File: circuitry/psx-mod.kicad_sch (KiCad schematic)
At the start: 57 parts, among them J1 2x3P, J2 1x6P, J3 1x6P, J4 1x6P, J5 USB 2.0 Type-C, Q1 SI2302, Q2 SI2302, SW1 RESET, U1 TPS78318DDCT, U2 CDCE925PWR, U3 74HC04, U4 ATmega328P-A, U5 USBLC6-2SC6, U6 CH340G, Y1 16MHz, Y2 27MHz, Y3 12MHz

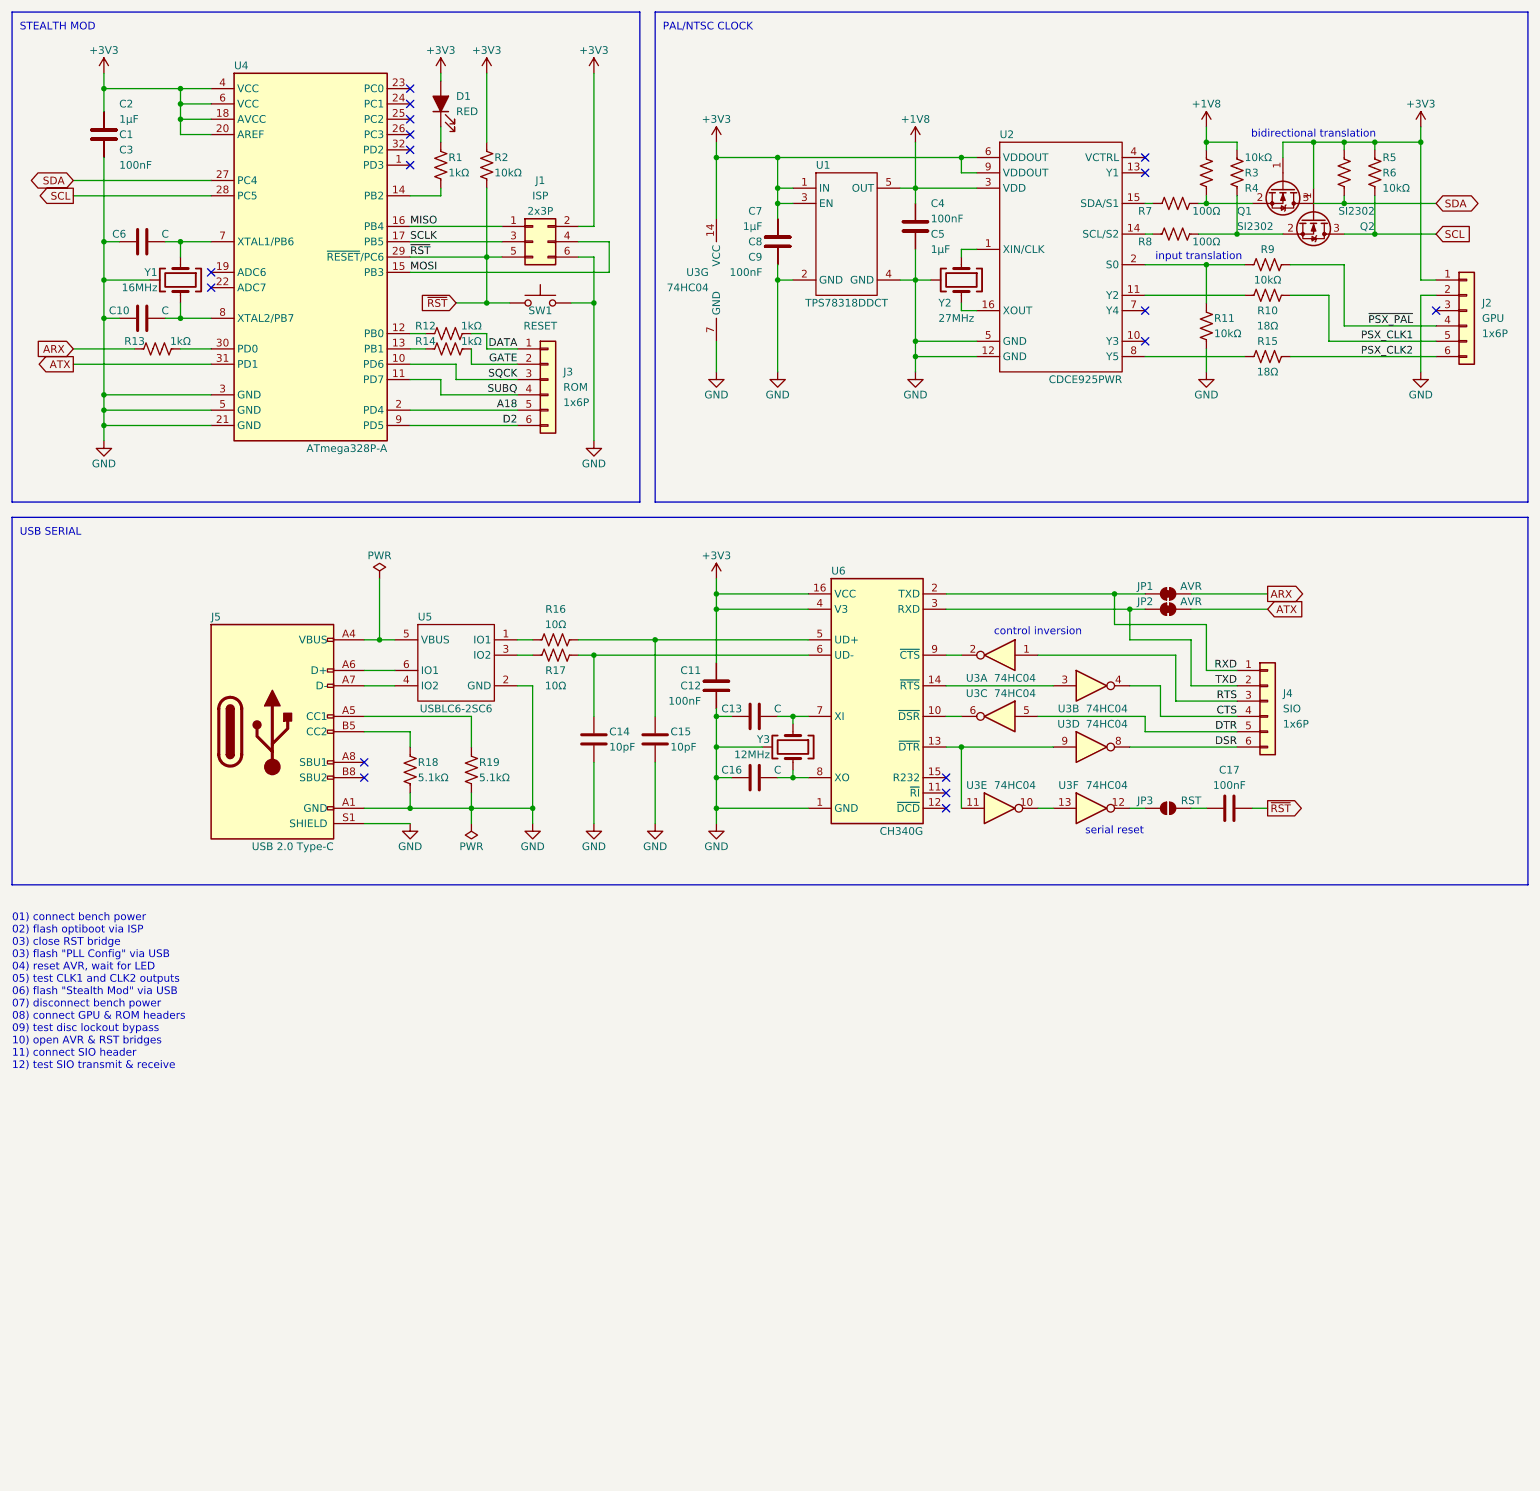
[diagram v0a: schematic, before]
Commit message: Completed schematic and layout (badly).
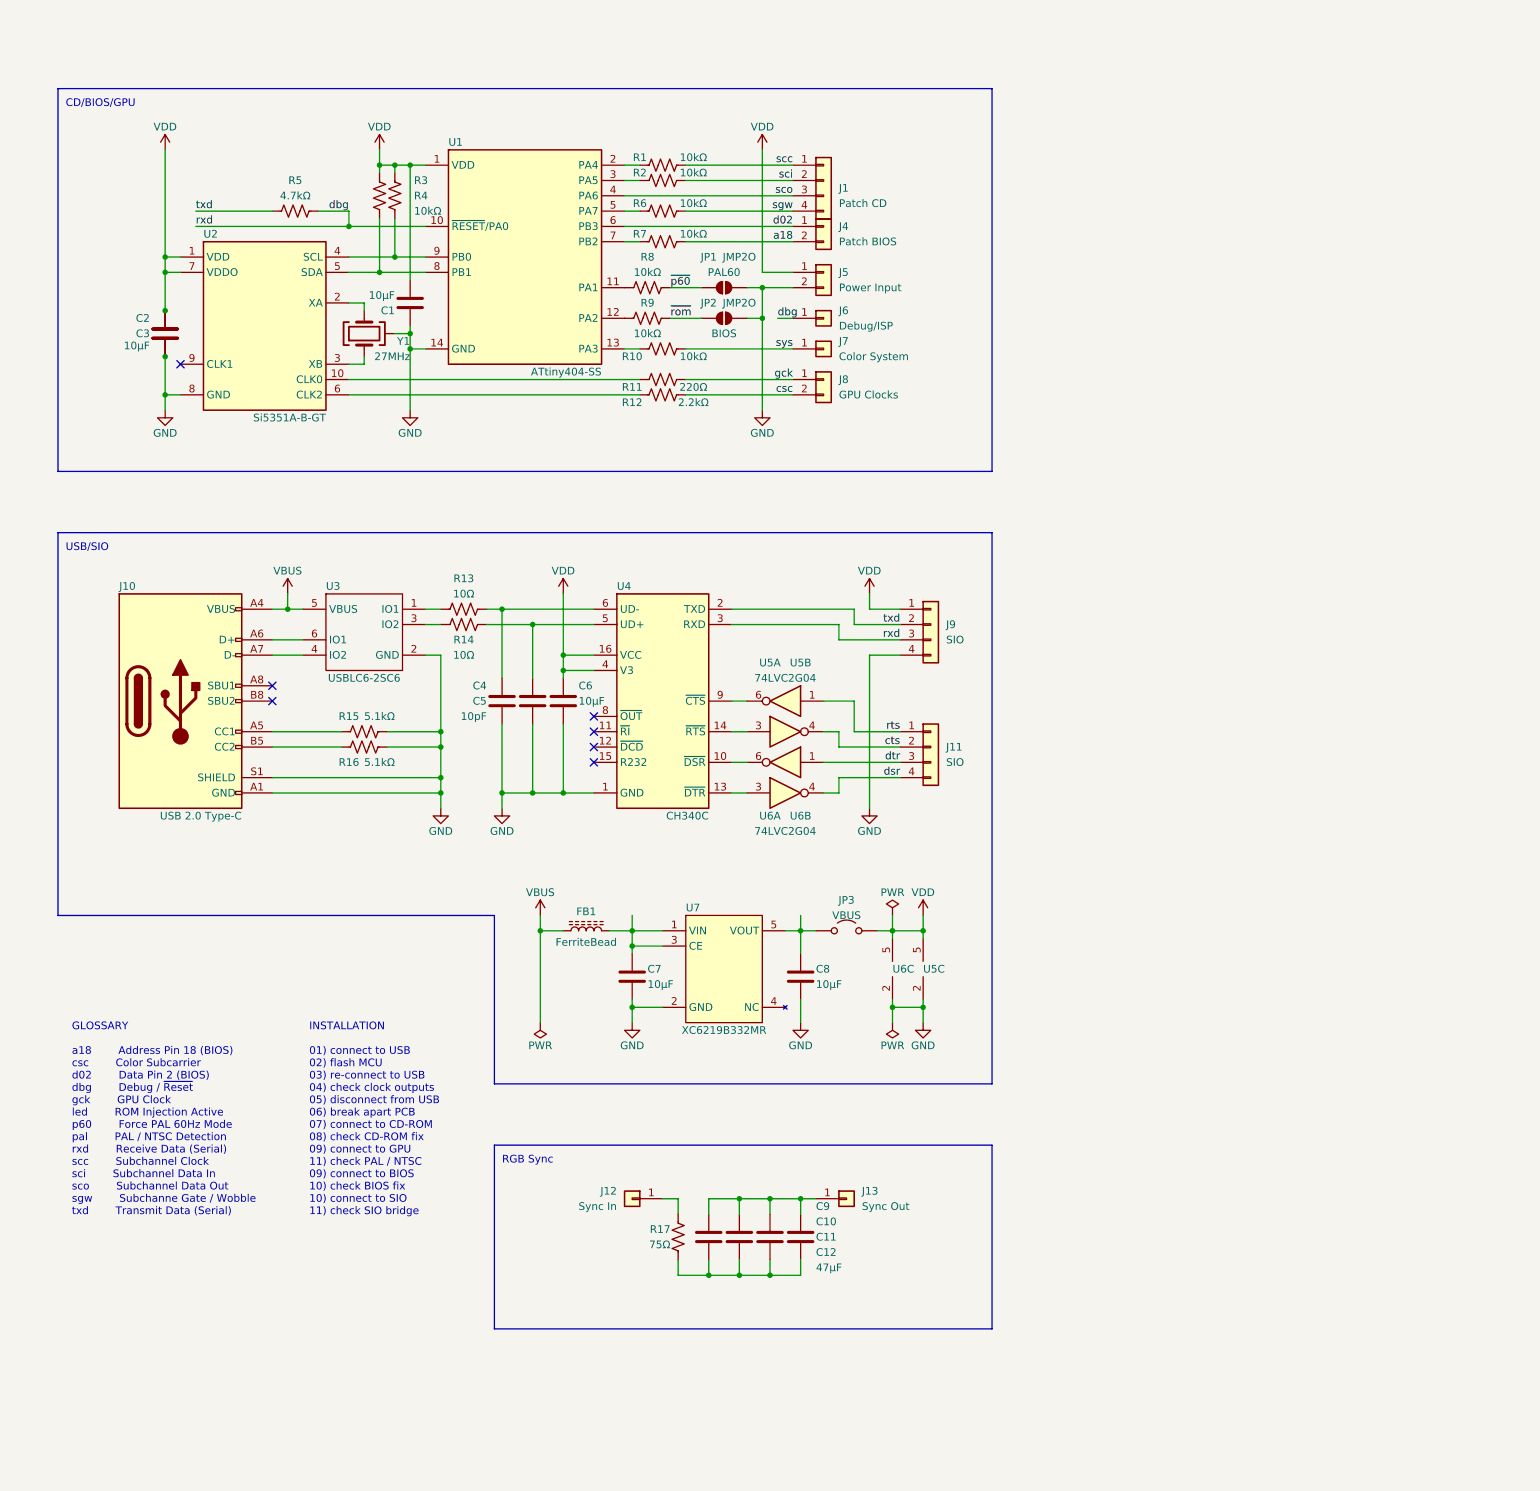
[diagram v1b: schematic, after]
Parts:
- removed C13, C16: C, Capacitor_SMD:C_0805_2012Metric_Pad1.18x1.45mm_HandSolder, symbol Device:C
- removed C14, C15: 10pF, Capacitor_SMD:C_0805_2012Metric_Pad1.18x1.45mm_HandSolder, symbol Device:C
- removed C17: 100nF, Capacitor_SMD:C_0805_2012Metric_Pad1.18x1.45mm_HandSolder, symbol Device:C
- removed D1: RED, Capacitor_SMD:C_0805_2012Metric_Pad1.18x1.45mm_HandSolder, symbol Device:LED_Filled
- removed J1: 2x3P, PSX_Mod:CONN-SMD_POGO-ISP, symbol Connector_Generic:Conn_02x03_Odd_Even
- removed J2, J3, J4: 1x6P, PSX_Mod:CONN-PH 1x06_P2.00mm_Horizontal, symbol Connector_Generic:Conn_01x06
- removed J5: USB 2.0 Type-C, PSX_Mod:CONN-SMD_HX-TYPE-C-16PIN, symbol PSX_Mod:USB_C_Receptacle_USB2.0_16P
- removed JP1, JP2: SolderJumper_2_Bridged, Jumper:SolderJumper-2_P1.3mm_Bridged2Bar_RoundedPad1.0x1.5mm, symbol Jumper:SolderJumper_2_Bridged
- removed JP3: SolderJumper_2_Open, Jumper:SolderJumper-2_P1.3mm_Open_RoundedPad1.0x1.5mm, symbol Jumper:SolderJumper_2_Open
- removed Q1, Q2: SI2302, Package_TO_SOT_SMD:SOT-23_Handsoldering, symbol Ashlyns_Symbols:SI2302
- removed R18, R19: 5.1kΩ, Resistor_SMD:R_0805_2012Metric_Pad1.20x1.40mm_HandSolder, symbol Device:R_US
- removed SW1: RESET, Button_Switch_SMD:SW_Push_1P1T_NO_6x6mm_H9.5mm, symbol Switch:SW_Push
- removed U1: TPS78318DDCT, Package_TO_SOT_SMD:SOT-23-5, symbol PSX_Mod:TPS78318DDCT
- removed U2: CDCE925PWR, Package_SO:TSSOP-16_4.4x5mm_P0.65mm, symbol PSX_Mod:CDCE925PWR
- removed U3: 74HC04, Package_SO:SOIC-14_3.9x8.7mm_P1.27mm, symbol PSX_Mod:74HC04
- removed U4: ATmega328P-A, Package_QFP:TQFP-32_7x7mm_P0.8mm, symbol PSX_Mod:ATmega328P-A
- removed U5: USBLC6-2SC6, Package_TO_SOT_SMD:SOT-23-6, symbol PSX_Mod:USBLC6_2SC6
- removed U6: CH340G, Package_SO:SOIC-16_3.9x9.9mm_P1.27mm, symbol PSX_Mod:CH340G
- removed Y2: 27MHz, Crystal:Crystal_SMD_3225-4Pin_3.2x2.5mm_HandSoldering, symbol PSX_Mod:Crystal
- removed Y3: 12MHz, Crystal:Crystal_SMD_3225-4Pin_3.2x2.5mm_HandSoldering, symbol PSX_Mod:Crystal
- added FB1: FerriteBead, Inductor_SMD:L_1206_3216Metric_Pad1.42x1.75mm_HandSolder, symbol Device:L_Ferrite
- added J1, J11, J9: Conn_01x04, PSX_Mod:CONN-SMD_4P, symbol Connector_Generic:Conn_01x04
- added J10: USB 2.0 Type-C, PSX_Mod:CONN-SMD_HX-TYPE-C-16PIN, symbol PSX_Mod:USB_C_Receptacle_USB2.0_16P
- added J12, J13, J6, J7: Conn_01x01, PSX_Mod:CONN-SMD_1P, symbol Connector_Generic:Conn_01x01
- added J4, J5, J8: Conn_01x02, PSX_Mod:CONN-SMD_2P, symbol Connector_Generic:Conn_01x02
- added JP1, JP2: JMP2O, Jumper:SolderJumper-2_P1.3mm_Open_RoundedPad1.0x1.5mm, symbol Jumper:SolderJumper_2_Open
- added JP3: Jumper_2_Open, Jumper:SolderJumper-2_P1.3mm_Open_RoundedPad1.0x1.5mm, symbol Jumper:Jumper_2_Open
- added U1: ATtiny404-SS, Package_SO:SOIC-14_3.9x8.7mm_P1.27mm, symbol PSX_Mod:ATtiny404-SS
- added U2: Si5351A-B-GT, Package_SO:MSOP-10_3x3mm_P0.5mm, symbol PSX_Mod:Si5351A-B-GT
- added U3: USBLC6-2SC6, Package_TO_SOT_SMD:SOT-23-6, symbol PSX_Mod:USBLC6_2SC6
- added U4: CH340C, Package_SO:SOIC-16_3.9x9.9mm_P1.27mm, symbol PSX_Mod:CH340C
- added U5, U6: 74LVC2G04, Package_TO_SOT_SMD:SOT-23-6, symbol PSX_Mod:74LVC2G04
- added U7: XC6219B332MR, Package_TO_SOT_SMD:SOT-23-5, symbol PSX_Mod:XC6219B332MR
- C1: value 100nF -> 10µF; footprint Capacitor_SMD:C_0805_2012Metric_Pad1.18x1.45mm_HandSolder -> Capacitor_SMD:C_0603_1608Metric_Pad1.08x0.95mm_HandSolder
- C10: value C -> 47µF; footprint Capacitor_SMD:C_0805_2012Metric_Pad1.18x1.45mm_HandSolder -> Capacitor_SMD:C_1206_3216Metric_Pad1.33x1.80mm_HandSolder
- C11: value 100nF -> 47µF; footprint Capacitor_SMD:C_0805_2012Metric_Pad1.18x1.45mm_HandSolder -> Capacitor_SMD:C_1206_3216Metric_Pad1.33x1.80mm_HandSolder; Proximity USB -> (none)
- C12: value 100nF -> 47µF; footprint Capacitor_SMD:C_0805_2012Metric_Pad1.18x1.45mm_HandSolder -> Capacitor_SMD:C_1206_3216Metric_Pad1.33x1.80mm_HandSolder; Proximity Inverter -> (none)
- C2: value 1µF -> 10µF; footprint Capacitor_SMD:C_0805_2012Metric_Pad1.18x1.45mm_HandSolder -> Capacitor_SMD:C_0603_1608Metric_Pad1.08x0.95mm_HandSolder; Proximity (none) -> PLL
- C3: value 100nF -> 10µF; footprint Capacitor_SMD:C_0805_2012Metric_Pad1.18x1.45mm_HandSolder -> Capacitor_SMD:C_0603_1608Metric_Pad1.08x0.95mm_HandSolder; Proximity (none) -> PLL
- C4: value 100nF -> 10pF; footprint Capacitor_SMD:C_0805_2012Metric_Pad1.18x1.45mm_HandSolder -> Capacitor_SMD:C_0603_1608Metric_Pad1.08x0.95mm_HandSolder; Proximity PLL -> (none)
- C5: value 1µF -> 10pF; footprint Capacitor_SMD:C_0805_2012Metric_Pad1.18x1.45mm_HandSolder -> Capacitor_SMD:C_0603_1608Metric_Pad1.08x0.95mm_HandSolder; Proximity VREG -> (none)
- C6: value C -> 10µF; footprint Capacitor_SMD:C_0805_2012Metric_Pad1.18x1.45mm_HandSolder -> Capacitor_SMD:C_0603_1608Metric_Pad1.08x0.95mm_HandSolder
- C7: value 1µF -> 10µF; footprint Capacitor_SMD:C_0805_2012Metric_Pad1.18x1.45mm_HandSolder -> Capacitor_SMD:C_0603_1608Metric_Pad1.08x0.95mm_HandSolder; Proximity VREG -> (none)
- C8: value 100nF -> 10µF; footprint Capacitor_SMD:C_0805_2012Metric_Pad1.18x1.45mm_HandSolder -> Capacitor_SMD:C_0603_1608Metric_Pad1.08x0.95mm_HandSolder; Proximity PLL -> (none)
- C9: value 100nF -> 47µF; footprint Capacitor_SMD:C_0805_2012Metric_Pad1.18x1.45mm_HandSolder -> Capacitor_SMD:C_1206_3216Metric_Pad1.33x1.80mm_HandSolder; Proximity PLL -> (none)
- R1: value 1kΩ -> 10kΩ; footprint Resistor_SMD:R_0805_2012Metric_Pad1.20x1.40mm_HandSolder -> Resistor_SMD:R_0603_1608Metric_Pad0.98x0.95mm_HandSolder
- R10: value 18Ω -> 10kΩ; footprint Resistor_SMD:R_0805_2012Metric_Pad1.20x1.40mm_HandSolder -> Resistor_SMD:R_0603_1608Metric_Pad0.98x0.95mm_HandSolder
- R11: value 10kΩ -> 220Ω; footprint Resistor_SMD:R_0805_2012Metric_Pad1.20x1.40mm_HandSolder -> Resistor_SMD:R_0603_1608Metric_Pad0.98x0.95mm_HandSolder
- R12: value 1kΩ -> 2.2kΩ; footprint Resistor_SMD:R_0805_2012Metric_Pad1.20x1.40mm_HandSolder -> Resistor_SMD:R_0603_1608Metric_Pad0.98x0.95mm_HandSolder
- R13, R14: value 1kΩ -> 10Ω; footprint Resistor_SMD:R_0805_2012Metric_Pad1.20x1.40mm_HandSolder -> Resistor_SMD:R_0603_1608Metric_Pad0.98x0.95mm_HandSolder
- R15: value 18Ω -> 5.1kΩ; footprint Resistor_SMD:R_0805_2012Metric_Pad1.20x1.40mm_HandSolder -> Resistor_SMD:R_0603_1608Metric_Pad0.98x0.95mm_HandSolder
- R16: value 10Ω -> 5.1kΩ; footprint Resistor_SMD:R_0805_2012Metric_Pad1.20x1.40mm_HandSolder -> Resistor_SMD:R_0603_1608Metric_Pad0.98x0.95mm_HandSolder
- R17: value 10Ω -> 75Ω; footprint Resistor_SMD:R_0805_2012Metric_Pad1.20x1.40mm_HandSolder -> Resistor_SMD:R_1206_3216Metric_Pad1.30x1.75mm_HandSolder
- R2, R3, R4, R6, R9: footprint Resistor_SMD:R_0805_2012Metric_Pad1.20x1.40mm_HandSolder -> Resistor_SMD:R_0603_1608Metric_Pad0.98x0.95mm_HandSolder
- R5: value 10kΩ -> 4.7kΩ; footprint Resistor_SMD:R_0805_2012Metric_Pad1.20x1.40mm_HandSolder -> Resistor_SMD:R_0603_1608Metric_Pad0.98x0.95mm_HandSolder
- R7, R8: value 100Ω -> 10kΩ; footprint Resistor_SMD:R_0805_2012Metric_Pad1.20x1.40mm_HandSolder -> Resistor_SMD:R_0603_1608Metric_Pad0.98x0.95mm_HandSolder
- Y1: value 16MHz -> 27MHz; footprint Crystal:Crystal_SMD_3225-4Pin_3.2x2.5mm_HandSoldering -> Crystal:Crystal_SMD_3225-4Pin_3.2x2.5mm; Load (none) -> 10pF
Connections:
- net PSX_CLK2 is gone; now on net GND: R15.2
- net GND: now also C6.2, R16.2, J10.A1 (GND), J10.A12 (GND), J10.B1 (GND), J10.B12 (GND), J10.S1 (SHIELD), J5.2 (Pin_2), J9.4 (Pin_4), JP1.2 (B), JP2.2 (B), U1.14 (GND), U2.8 (GND), U3.2 (GND), U4.1 (GND), U5.2 (GND), U6.2 (GND), U7.2 (GND); no longer C10.1, C11.2, C12.2, C6.1, C9.2, R11.2
- net at R10.1: now also U1.13 (PA3)
- net at R11.1: now also U2.10 (CLK0); no longer R9.1
- net at R12.1: now also U2.6 (CLK2)
- net at R14.1: now also U3.3 (IO2)
- net scc: now reaches R1.2
- net scc: now also J1.1 (Pin_1)
- net at R13.2: now also C4.1, U4.6 (UD-)
- net at Y1.1: now also U2.3 (XB); no longer C6.2
- net at C10.2: now also C11.2, C12.2, C9.2, R17.1; no longer Y1.3
- net at R7.1: now also U1.7 (PB2)
- net at R3.2: now also U1.8 (PB1), U2.5 (SDA); no longer R7.2
- net at R8.1: now also U1.11 (PA1)
- net at R4.2: now also U1.9 (PB0), U2.4 (SCL); no longer R8.2
- net at R1.1: now also U1.2 (PA4)
- net at R15.1: now also J10.A5 (CC1)
- net at R16.1: now also J10.B5 (CC2)
- net at R17.2: now also J12.1 (Pin_1)
- net +1V8 renamed VDD
- net VDD: now also C1.1, C2.1, C3.1, C6.1, J5.1 (Pin_1), J9.1 (Pin_1), JP3.2 (B), U1.1 (VDD), U2.1 (VDD), U2.7 (VDDO), U4.16 (VCC), U4.4 (V3), U5.5 (VCC), U6.5 (VCC); no longer C4.1, C5.1
- removed net +3V3: C1.1, C11.1, C12.1, C2.1, C3.1, C7.1, C8.1, C9.1, R2.1, R5.1, R6.1
- net ARX: no longer names the net of R13.1
- net ARX: now also U3.1 (IO1)
- net DATA renamed csc
- net csc: now also J8.2 (Pin_2)
- net GATE: no longer names the net of R14.2
- net GATE: now also C5.1, U4.5 (UD+)
- net PSX_CLK1 renamed sys
- net sys: now also J7.1 (Pin_1)
- net SCL renamed sgw
- net sgw: now also J1.4 (Pin_4)
- net SDA renamed dbg
- net dbg: now also J6.1 (Pin_1), J9.3 (Pin_3), U1.10 (~{RESET}/PA0), U4.3 (RXD)
- net ~{PSX_PAL} renamed ~{rom}
- net ~{rom}: now also JP2.1 (A)
- net ~{RST} renamed sci
- net sci: now also J1.2 (Pin_2)
- new net: U4.10 (~{DSR}), U6.6 (~{Y1})
- new net: U4.13 (~{DTR}), U6.3 (A2)
- new net: U4.14 (~{RTS}), U5.3 (A2)
- new net: U4.9 (~{CTS}), U5.6 (~{Y1})
- new net: C10.1, C11.1, C12.1, C9.1, J13.1 (Pin_1)
- new net: C7.1, FB1.2, U7.1 (VIN), U7.3 (CE)
- new net: C8.1, JP3.1 (A), U7.5 (VOUT)
- new net: R9.1, U1.12 (PA2)
- new net: R2.1, U1.3 (PA5)
- new net: R6.1, U1.5 (PA7)
- new net: J10.A7 (D-), J10.B7 (D-), U3.4 (IO2)
- new net: J10.A6 (D+), J10.B6 (D+), U3.6 (IO1)
- new net: U2.2 (XA), Y1.3
- new net VBUS: FB1.1, J10.A4 (VBUS), J10.A9 (VBUS), J10.B4 (VBUS), J10.B9 (VBUS), U3.5 (VBUS)
- new net a18: J4.2 (Pin_2), R7.2
- new net cts: J11.2 (Pin_2), U5.4 (~{Y2})
- new net d02: J4.1 (Pin_1), U1.6 (PB3)
- new net dsr: J11.4 (Pin_4), U6.4 (~{Y2})
- new net dtr: J11.3 (Pin_3), U6.1 (A1)
- new net gck: J8.1 (Pin_1), R11.2
- new net rts: J11.1 (Pin_1), U5.1 (A1)
- new net sco: J1.3 (Pin_3), U1.4 (PA6)
- new net txd: J9.2 (Pin_2), R5.1, U4.2 (TXD)
- new net ~{p60}: JP1.1 (A), R8.2
- no-connect marks 18 -> 7
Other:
- note added: "CD/BIOS/GPU"
- note added: "RGB Sync"
- note added: "USB/SIO"
- note removed: "01) connect bench power 02) flash optiboot via ISP 03) close RST bridge 03) flash "PLL Config" via USB 04) reset AVR, wait for LED 05) test CLK1 and CLK2 outputs 06) flash "Stealth Mod" via USB 07) disconnect bench power 08) connect GPU & ROM headers 09) test disc lockout bypass 10) open AVR & RST bridges 11) connect SIO header 12) test SIO transmit & receive"
- note removed: "PAL/NTSC CLOCK"
- note removed: "STEALTH MOD"
- note removed: "USB SERIAL"
- note removed: "bidirectional translation"
- note removed: "control inversion"
- note removed: "input translation"
- note removed: "serial reset"
- title: PSX-MOD -> PSX Modchip
